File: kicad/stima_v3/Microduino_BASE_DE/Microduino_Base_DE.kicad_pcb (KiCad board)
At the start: 2 copper layers, 25.5 x 27.9 mm, 4 parts, among them P1 CONN_01X02, P2 CONN_01X04, P3 CONN_1x27

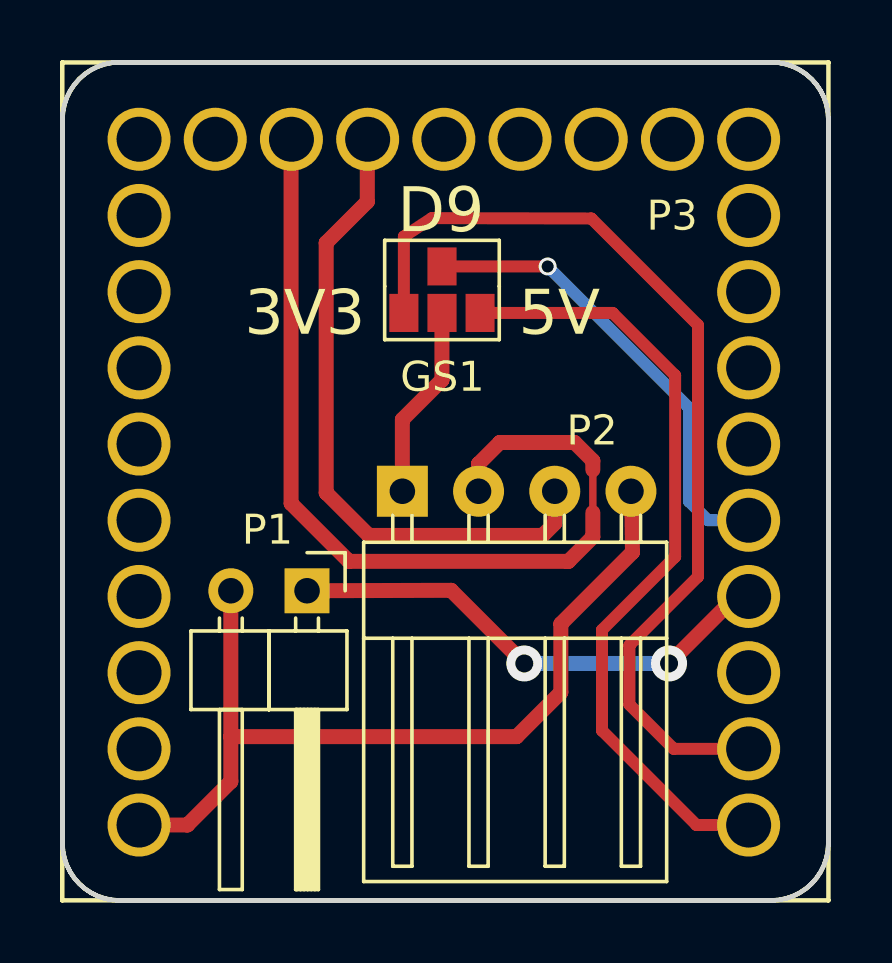
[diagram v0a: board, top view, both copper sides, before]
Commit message: reapload kicad scheme
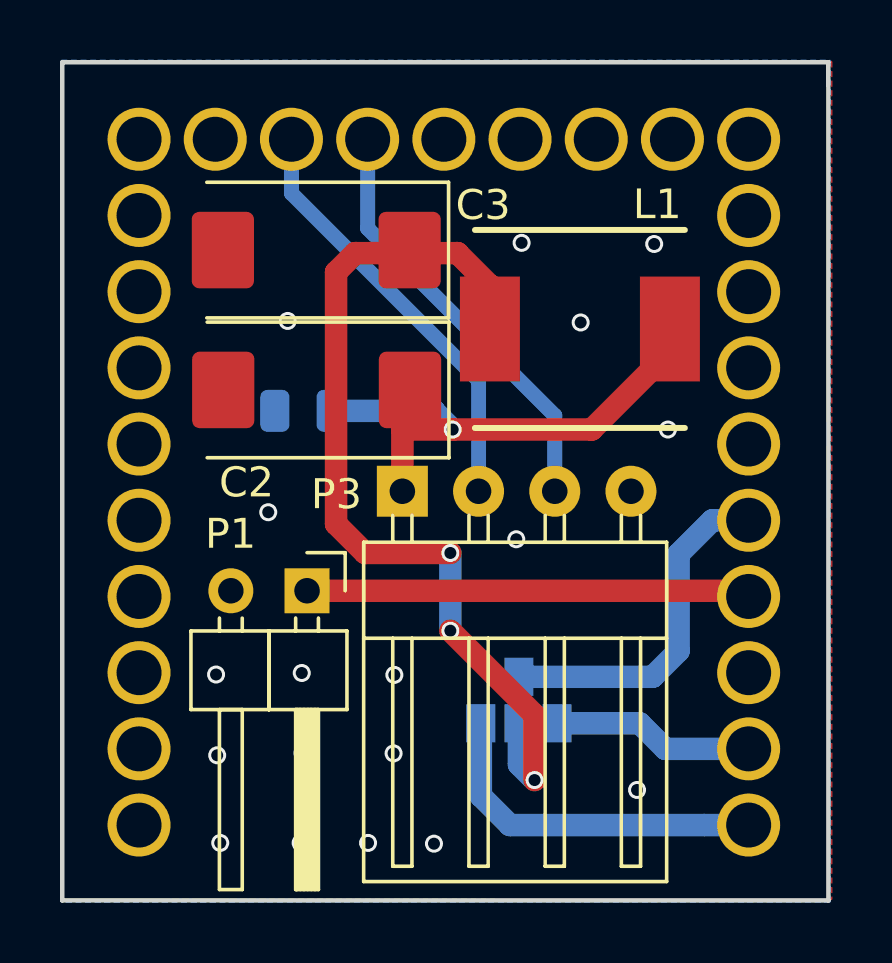
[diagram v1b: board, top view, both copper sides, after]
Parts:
- added C1: 100nF, Capacitor_SMD:C_0805_2012Metric, B.Cu at (146.7, 74.4)
- added C2: 330uF, Capacitor_Tantalum_SMD:CP_EIA-7343-43_Kemet-X, F.Cu at (147.2, 73.7)
- added C3: 330uF, Capacitor_Tantalum_SMD:CP_EIA-7343-43_Kemet-X, F.Cu at (147.2, 69.0)
- added L1: 10uH, SamacSys_Parts:FDSD0630H100MP3, F.Cu at (156.0, 71.6)
- GS1: moved to B.Cu
- moved GS1 13.9 mm to (153.9, 84.8)
- renumbered P3 to P2, P2 to P3
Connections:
- GS1 pad 2: Net-(GS1-Pad2) -> Net-(C3-Pad1)
- P3 pad 1: Net-(GS1-Pad2) -> Net-(C1-Pad2)
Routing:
- net Net-(C3-Pad1): track 0.00 -> 30.7 mm, vias 0 -> 3
- net GND: track 29.3 -> 0.00 mm, vias 0 -> 18
- net +3V3: track 32.2 -> 6.74 mm
- net Net-(C1-Pad2): track 0.00 -> 18.5 mm, vias 0 -> 1
- net /SCL: track 31.1 -> 14.3 mm
- net +5V: track 27.2 -> 12.5 mm
- net /SDA: track 21.8 -> 14.3 mm
- net Net-(GS1-Pad2): track 6.39 -> 0.00 mm
- net /D9: track 15.5 -> 11.7 mm, vias 1 -> 0
- net /D8: track 16.9 -> 14.8 mm, vias 2 -> 0
- added copper zone on B.Cu, net GND
- added copper zone on F.Cu, net GND
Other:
- outline, holes or cut-outs redrawn
